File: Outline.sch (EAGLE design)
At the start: 47 parts, among them CN1 0675031020, IC1 ATXMEGA32A4U-AU, IC2 ST1480ACDR, J1 RJHSE5080, J2 J2, Q1 BC817-16, U1 NCP1117DTAG @ 3.3v, U2 NCP1117DTAG @ 12v

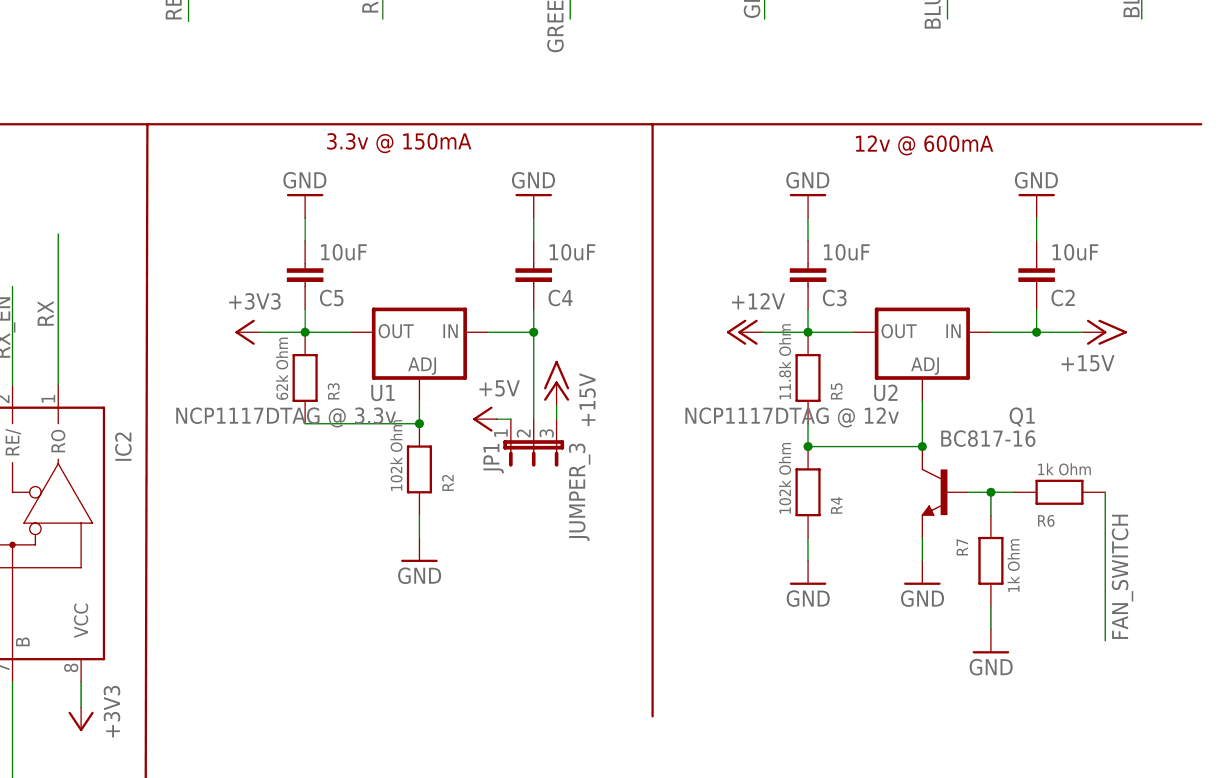
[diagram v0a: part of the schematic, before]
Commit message: Version 4
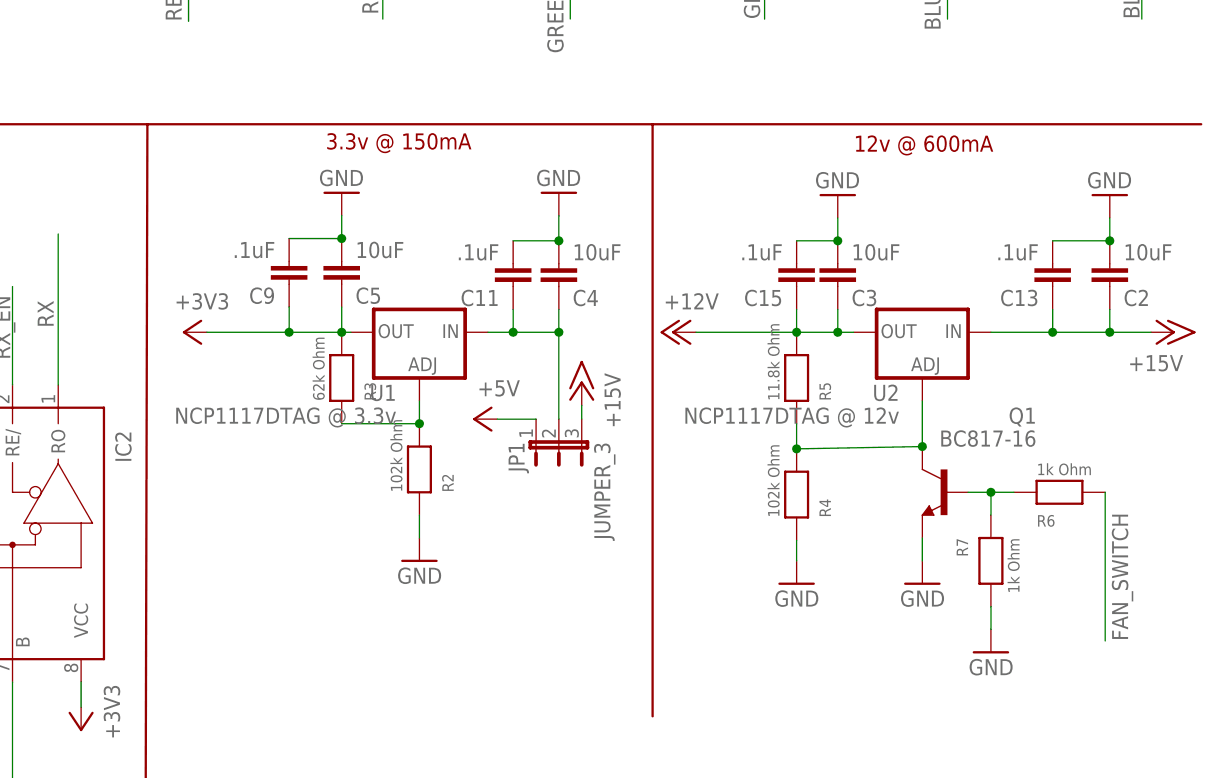
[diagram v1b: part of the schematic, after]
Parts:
- added C11, C13, C15, C9: .1uF, SparkFun:CAP0603-CAP
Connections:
- net +12V: now also C15.1
- net +15V: now also C13.1
- net +3V3: now also C9.1
- net GND: now also C11.2, C13.2, C15.2, C9.2
- net N$21: now also C11.1
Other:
- moved on the sheet: C2, C3, C4, C5, JP1, R3, R4, R5

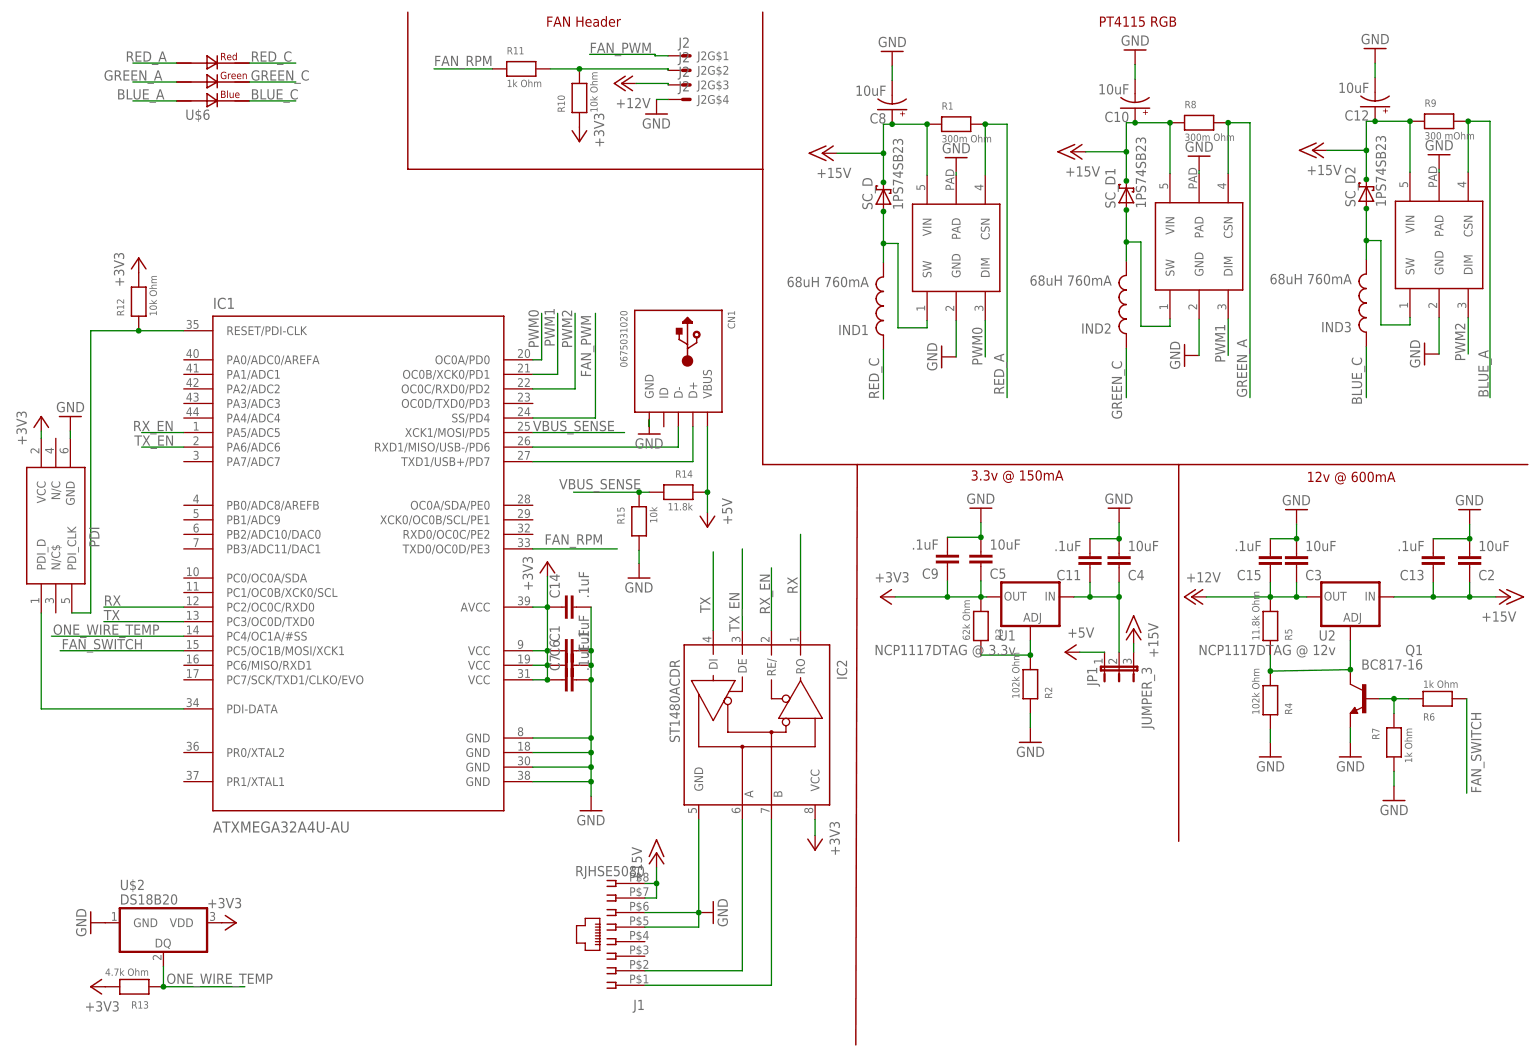
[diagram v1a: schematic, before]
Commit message: Version 4.1
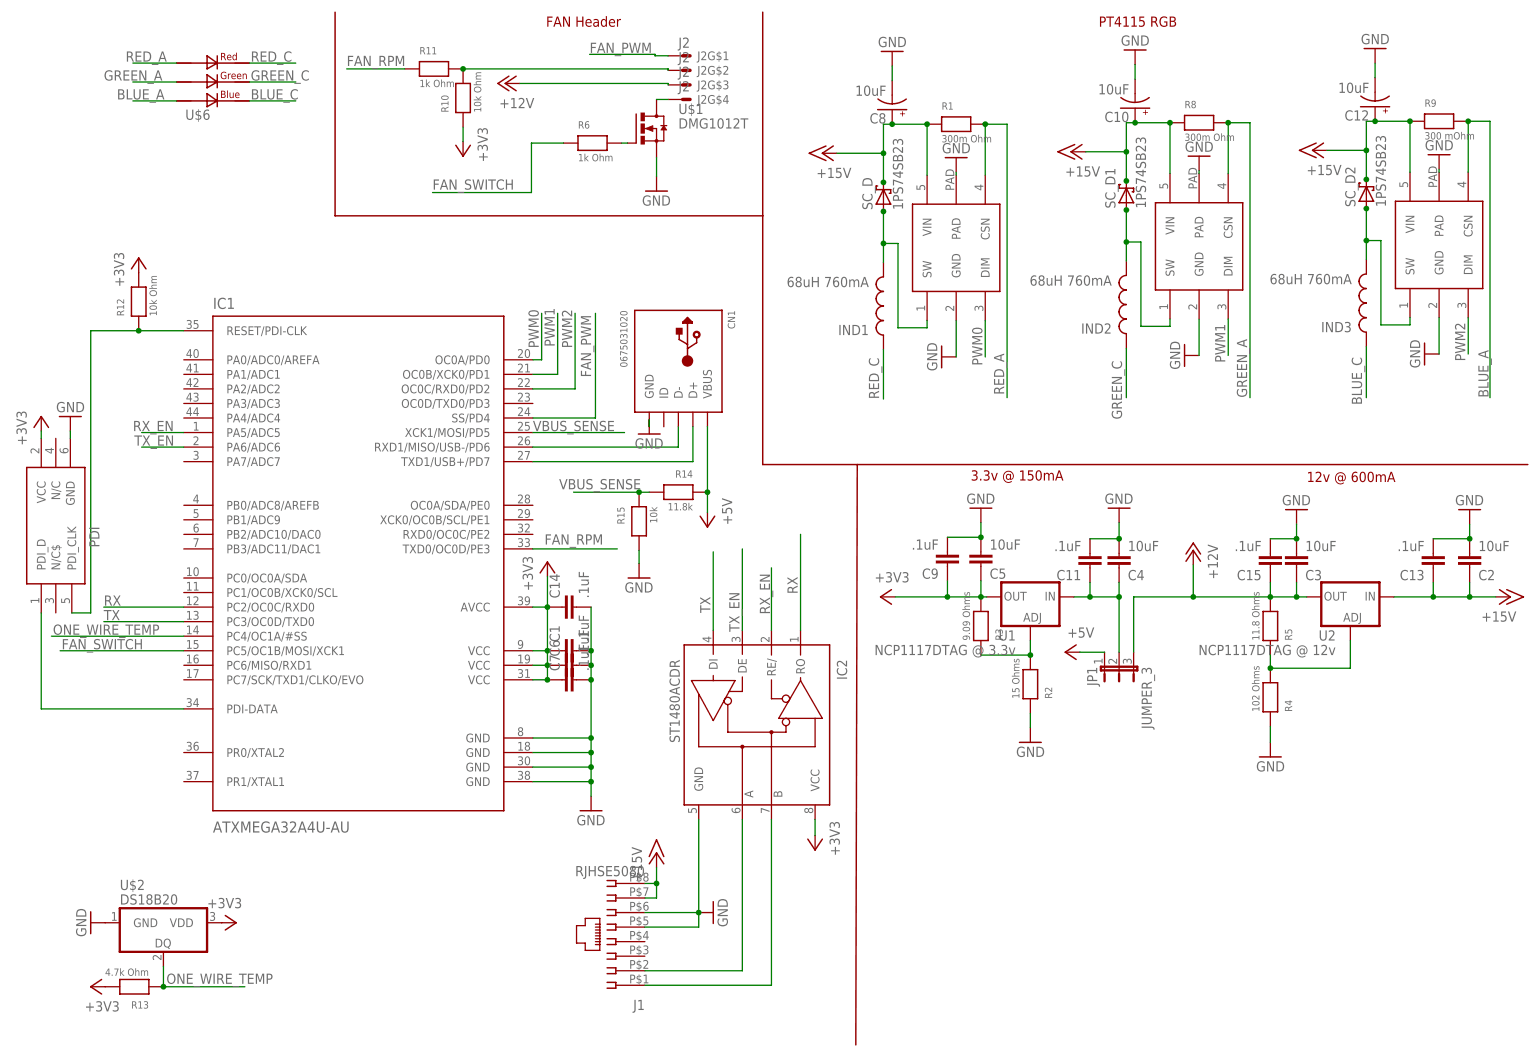
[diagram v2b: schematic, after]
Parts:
- removed Q1: BC817-16, dp_devices:TRANSISTOR_BJT_NPN-SOT-23-BEC
- removed R7: 1k Ohm, nonolith:RESISTOR0603
- added U$1: DMG1012T, TechIsCool:DMG1012T
- R2: value 102k Ohm -> 15 Ohms
- R3: value 62k Ohm -> 9.09 Ohms
- R4: value 102k Ohm -> 102 Ohms
- R5: value 11.8k Ohm -> 11.8 Ohms
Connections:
- new net N$4: R6.2, U$1.G
- net +12V: now also JP1.3
- net +15V: no longer JP1.3
- net FAN_SWITCH: now also R6.1; no longer R6.2
- net GND: now also U$1.S; no longer J2G$4.S, Q1.E, R7.2
- net N$2: no longer Q1.C
- net N$3: now also J2G$4.S, U$1.D; no longer Q1.B, R6.1, R7.1
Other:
- moved on the sheet: R10, R11, R4, R6
